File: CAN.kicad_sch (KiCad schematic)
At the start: 6 parts

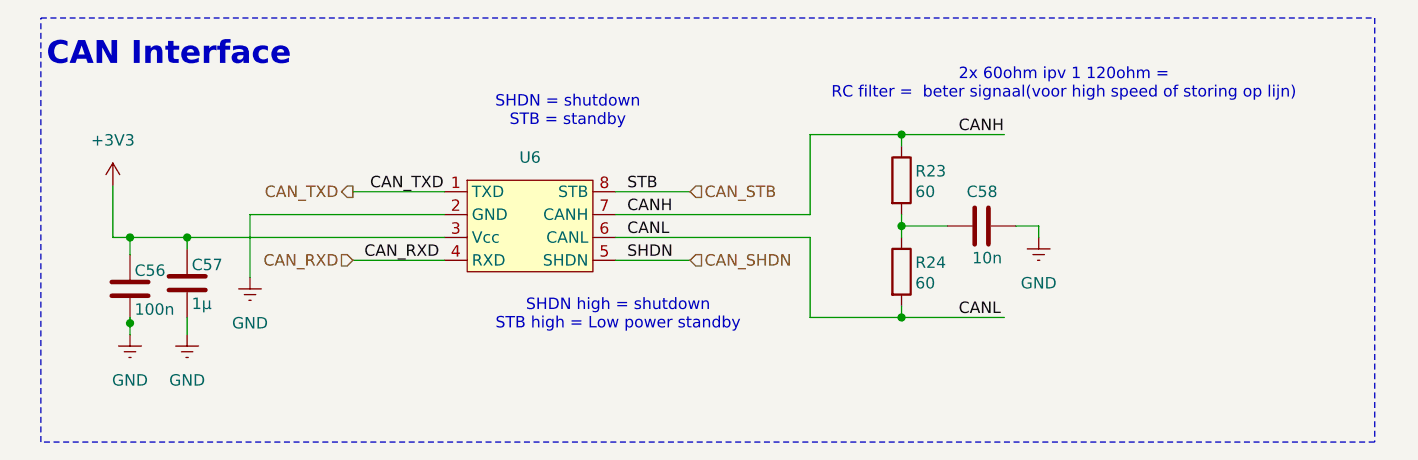
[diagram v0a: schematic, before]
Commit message: al de main blokken bij elkaar gezet op juiste plaats
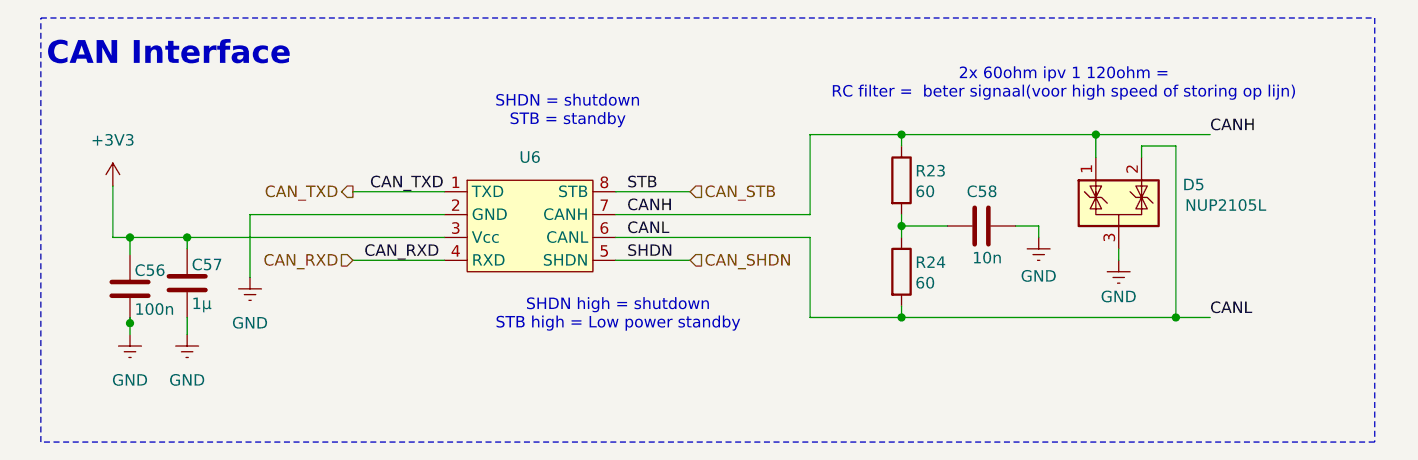
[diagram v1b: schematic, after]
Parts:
- added D5: NUP2105L, Package_TO_SOT_SMD:SOT-23, symbol Power_Protection:NUP2105L
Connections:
- net CANH: now also D5.1 (K)
- net CANL: now also D5.2 (K)
- net GND: now also D5.3 (A)
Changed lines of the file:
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@@
+	)
+	(junction
+		(at 205.74 88.9)
+		(diameter 0)
+		(color 0 0 0 0)
 	)
 	(junction
@@
 	)
 	(junction
+		(at 196.85 68.58)
+		(diameter 0)
+		(color 0 0 0 0)
+	)
+	(junction
 		(at 89.535 89.535)
 		(diameter 0)
@@
 	(wire
 		(pts
+			(xy 199.39 81.28) (xy 199.39 82.55)
+		)
+		(stroke
+			(width 0)
+			(type default)
+		)
+	)
+	(wire
+		(pts
 			(xy 87.63 80.01) (xy 89.535 80.01)
 		)
@@
 	(wire
 		(pts
+			(xy 201.93 69.85) (xy 201.93 71.12)
+		)
+		(stroke
+			(width 0)
+			(type default)
+		)
+	)
+	(wire
+		(pts
 			(xy 89.535 89.535) (xy 89.535 90.805)
 		)
@@
 	(wire
 		(pts
+			(xy 196.85 68.58) (xy 209.55 68.58)
+		)
+		(stroke
+			(width 0)
+			(type default)
+		)
+	)
+	(wire
+		(pts
 			(xy 175.26 78.74) (xy 180.34 78.74)
 		)
@@
 	(wire
 		(pts
+			(xy 205.74 69.85) (xy 205.74 88.9)
+		)
+		(stroke
+			(width 0)
+			(type default)
+		)
+	)
+	(wire
+		(pts
+			(xy 205.74 88.9) (xy 209.55 88.9)
+		)
+		(stroke
+			(width 0)
+			(type default)
+		)
+	)
+	(wire
+		(pts
+			(xy 196.85 68.58) (xy 196.85 71.12)
+		)
+		(stroke
+			(width 0)
+			(type default)
+		)
+	)
+	(wire
+		(pts
+			(xy 201.93 69.85) (xy 205.74 69.85)
+		)
+		(stroke
+			(width 0)
+			(type default)
+		)
+	)
+	(wire
+		(pts
 			(xy 95.885 88.9) (xy 95.885 90.805)
 		)
@@
 	(wire
 		(pts
-			(xy 175.26 68.58) (xy 186.69 68.58)
+			(xy 175.26 68.58) (xy 196.85 68.58)
 		)
 		(stroke
@@
 	(wire
 		(pts
-			(xy 175.26 88.9) (xy 186.69 88.9)
+			(xy 175.26 88.9) (xy 205.74 88.9)
 		)
 		(stroke
@@
 	)
 	(label "CANH"
-		(at 181.61 68.58 0)
+		(at 209.55 68.58 0)
 		(effects
 			(font
@@
 	)
 	(label "CANL"
-		(at 181.61 88.9 0)
+		(at 209.55 88.9 0)
 		(effects
 			(font
@@
 	)
 	(symbol
+		(lib_id "Power_Protection:NUP2105L")
+		(at 199.39 76.2 0)
+		(unit 1)
+		(body_style 1)
+		(exclude_from_sim no)
+		(in_bom yes)
+		(on_board yes)
+		(in_pos_files yes)
+		(dnp no)
+		(property "Reference" "D5"
+			(at 206.502 74.168 0)
+			(show_name no)
+			(do_not_autoplace no)
+			(effects
+				(font
+					(size 1.27 1.27)
+				)
+				(justify left)
+			)
+		)
+		(property "Value" "NUP2105L"
+			(at 206.756 76.454 0)
+			(show_name no)
+			(do_not_autoplace no)
+			(effects
+				(font
+					(size 1.27 1.27)
+				)
+				(justify left)
+			)
+		)
+		(property "Footprint" "Package_TO_SOT_SMD:SOT-23"
+			(at 205.105 77.47 0)
+			(hide yes)
+			(show_name no)
+			(do_not_autoplace no)
+			(effects
+				(font
+					(size 1.27 1.27)
+				)
+				(justify left)
+			)
+		)
+		(property "Datasheet" "https://www.onsemi.com/pub_link/Collateral/NUP2105L-D.PDF"
+			(at 202.565 73.025 0)
+			(hide yes)
+			(show_name no)
+			(do_not_autoplace no)
+			(effects
+				(font
+					(size 1.27 1.27)
+				)
+			)
+		)
+		(property "Description" "Dual Line CAN Bus Protector, 24Vrwm"
+			(at 199.39 76.2 0)
+			(hide yes)
+			(show_name no)
+			(do_not_autoplace no)
+			(effects
+				(font
+					(size 1.27 1.27)
+				)
+			)
+		)
+		(pin "1"
+		)
+		(pin "3"
+		)
+		(pin "2"
+		)
+		(instances
+			(project "ESC_PLC"
+				(path "/5bd3bb6f-fe53-443c-806c-077e2bbb5d14/fe40b710-6ad0-4f5f-80cc-5572b327525f"
+					(reference "D5")
+					(unit 1)
+				)
+			)
+		)
+	)
+	(symbol
 		(lib_id "power:GNDREF")
 		(at 102.87 84.455 0)
@@
 		(in_pos_files yes)
 		(dnp no)
-		(fields_autoplaced yes)
 		(property "Reference" "#PWR071"
 			(at 190.5 86.36 0)
@@
 		)
 		(property "Value" "GND"
-			(at 190.5 85.09 0)
+			(at 190.5 84.328 0)
 			(show_name no)
 			(do_not_autoplace no)
@@
 					(unit 1)
 				)
+			)
+		)
+	)
+	(symbol
+		(lib_id "power:GNDREF")
+		(at 199.39 82.55 0)
+		(unit 1)
+		(body_style 1)
+		(exclude_from_sim no)
+		(in_bom yes)
+		(on_board yes)
+		(in_pos_files yes)
+		(dnp no)
+		(property "Reference" "#PWR0105"
+			(at 199.39 88.9 0)
+			(hide yes)
+			(show_name no)
+			(do_not_autoplace no)
+			(effects
+				(font
+					(size 1.27 1.27)
+				)
+			)
+		)
+		(property "Value" "GND"
+			(at 199.39 86.614 0)
+			(show_name no)
+			(do_not_autoplace no)
+			(effects
+				(font
+					(size 1.27 1.27)
+				)
+			)
+		)
+		(property "Footprint" ""
+			(at 199.39 82.55 0)
+			(hide yes)
+			(show_name no)
+			(do_not_autoplace no)
+			(effects
+				(font
+					(size 1.27 1.27)
+				)
+			)
+		)
+		(property "Datasheet" ""
+			(at 199.39 82.55 0)
+			(hide yes)
+			(show_name no)
+			(do_not_autoplace no)
+			(effects
+				(font
+					(size 1.27 1.27)
+				)
+			)
+		)
+		(property "Description" "Power symbol creates a global label with name \"GNDREF\" , reference supply ground"
+			(at 199.39 82.55 0)
+			(hide yes)
+			(show_name no)
+			(do_not_autoplace no)
+			(effects
+				(font
+					(size 1.27 1.27)
+				)
+			)
+		)
+		(pin "1"
+		)
+		(instances
+			(project "ESC_PLC"
+				(path "/5bd3bb6f-fe53-443c-806c-077e2bbb5d14/fe40b710-6ad0-4f5f-80cc-5572b327525f"
+					(reference "#PWR0105")
+					(unit 1)
+				)
